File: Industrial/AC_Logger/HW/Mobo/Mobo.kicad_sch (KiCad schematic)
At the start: 5 parts

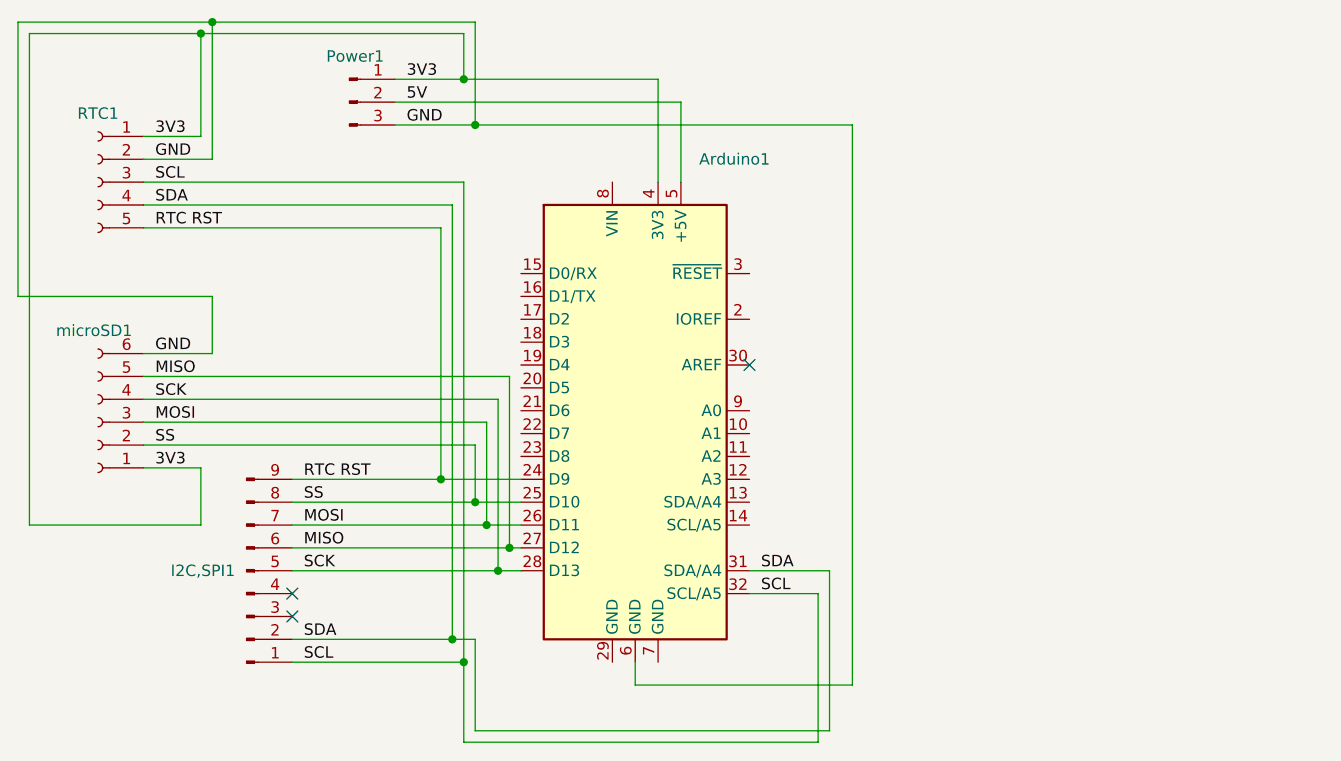
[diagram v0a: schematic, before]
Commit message: Last last edit to pcb
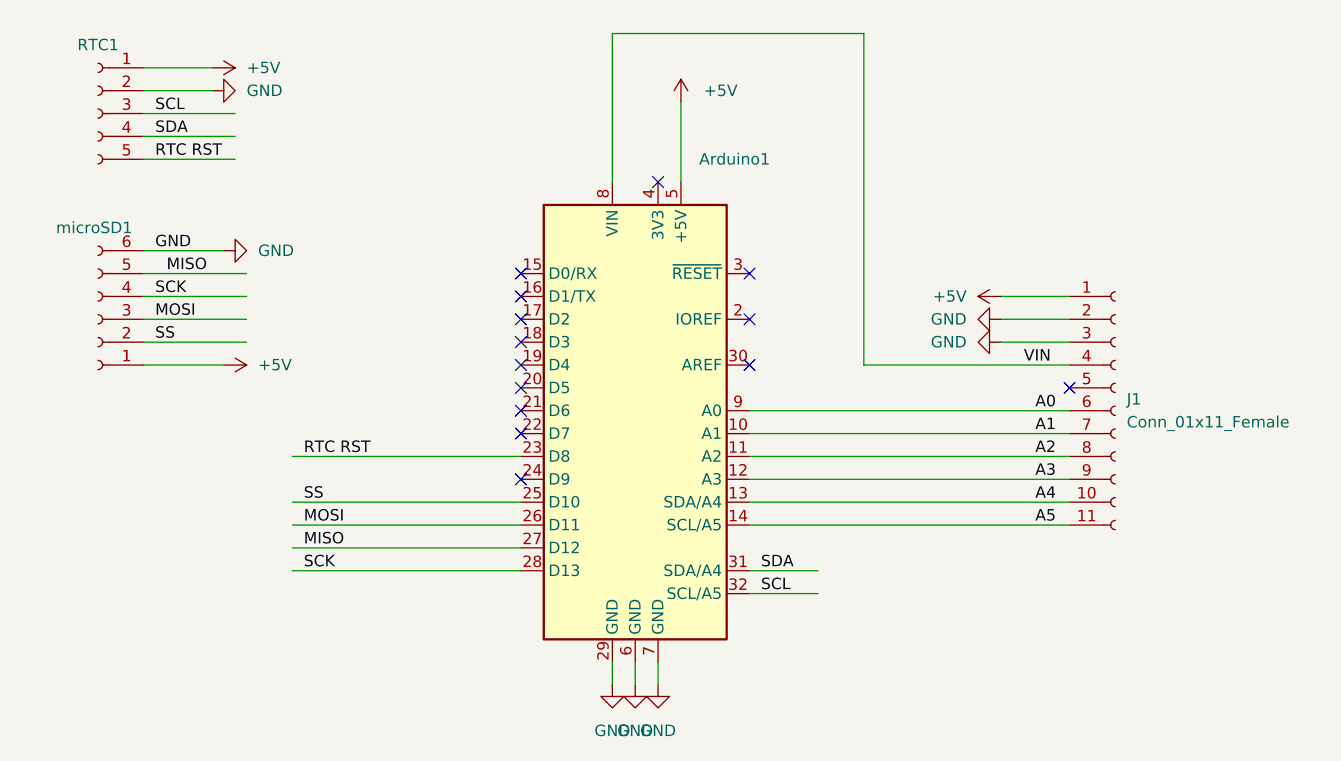
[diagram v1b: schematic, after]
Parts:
- removed I2C,SPI1: Conn_01x09_Male, Connector_PinHeader_2.54mm:PinHeader_1x09_P2.54mm_Vertical, symbol Connector:Conn_01x09_Male
- removed Power1: Conn_01x03_Male, Connector_PinHeader_2.54mm:PinHeader_1x03_P2.54mm_Vertical, symbol Connector:Conn_01x03_Male
- added J1: Conn_01x11_Female, Connector_PinSocket_2.54mm:PinSocket_1x11_P2.54mm_Vertical, symbol Connector:Conn_01x11_Female
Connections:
- net 5V is gone; now on net +5V: Arduino1.5 (+5V)
- net GND: now also Arduino1.29 (GND), Arduino1.7 (GND), J1.2 (Pin_2), J1.3 (Pin_3)
- net RTC RST: now also Arduino1.23 (D8); no longer Arduino1.24 (D9)
- net A1: now reaches Arduino1.10 (A1)
- net A1: now also J1.7 (Pin_7)
- net A2: now reaches Arduino1.11 (A2)
- net A2: now also J1.8 (Pin_8)
- net A3: now reaches Arduino1.12 (A3)
- net A3: now also J1.9 (Pin_9)
- net A4: now reaches Arduino1.13 (SDA/A4)
- net A4: now also J1.10 (Pin_10)
- net A5: now reaches Arduino1.14 (SCL/A5)
- net A5: now also J1.11 (Pin_11)
- net VIN: now reaches Arduino1.8 (VIN)
- net VIN: now also J1.4 (Pin_4)
- net A0: now reaches Arduino1.9 (A0)
- net A0: now also J1.6 (Pin_6)
- net 3V3 renamed +5V
- net +5V: now also J1.1 (Pin_1); no longer Arduino1.4 (3V3)
- no-connect marks 3 -> 14
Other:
- moved on the sheet: RTC1, microSD1
